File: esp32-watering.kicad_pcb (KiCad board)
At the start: 2 copper layers, 74.7 x 55.5 mm, 30 parts, among them J1 12V, J2 DS18B20, J3 FLOAT, J4 PUMP, J5 ZONE 1, J6 ZONE 2, J7 ZONE 3, K1 Pump Control, K2 Zone 1, K3 Zone 2, K4 Zone 3, Q1 2N3904, Q2 2N3904, Q3 2N3904, Q4 2N3904, U1 esp32-wemos-d1-mini, U2 TSR 1-2433

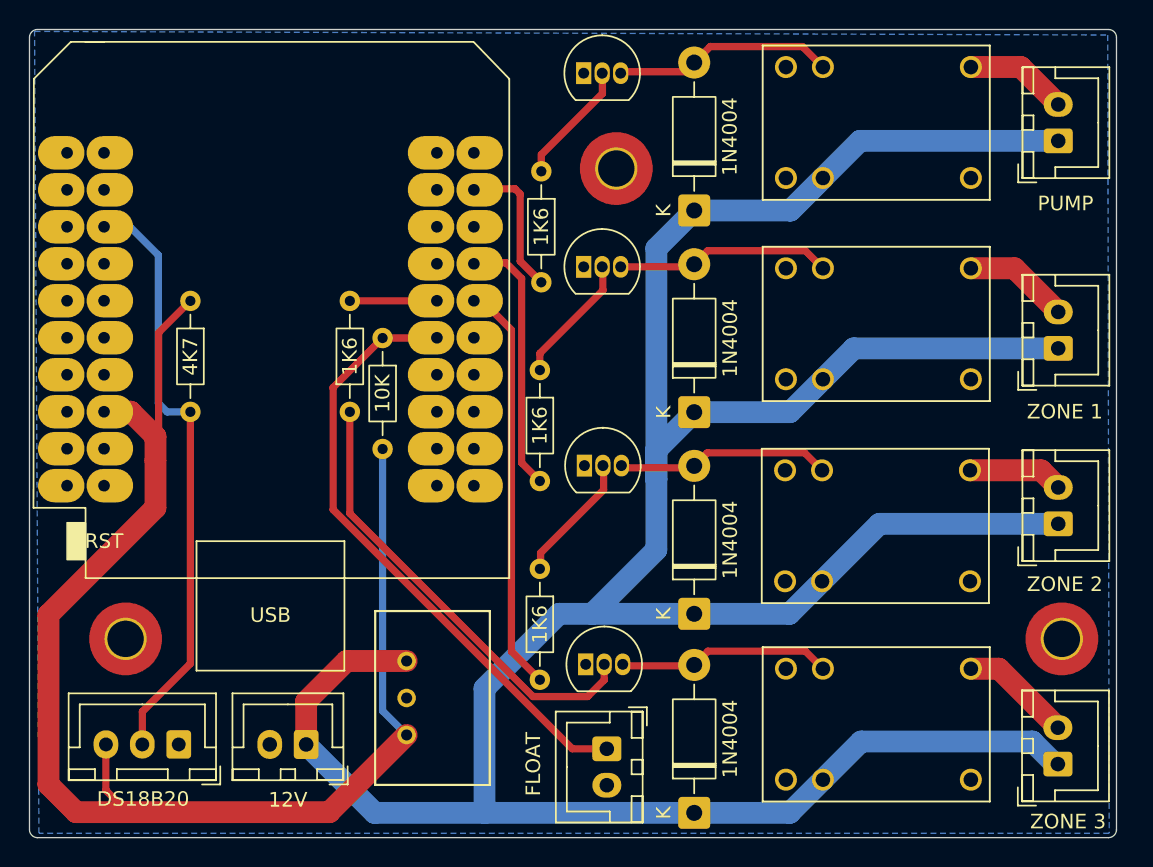
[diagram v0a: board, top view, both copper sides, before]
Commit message: Fix edge cut
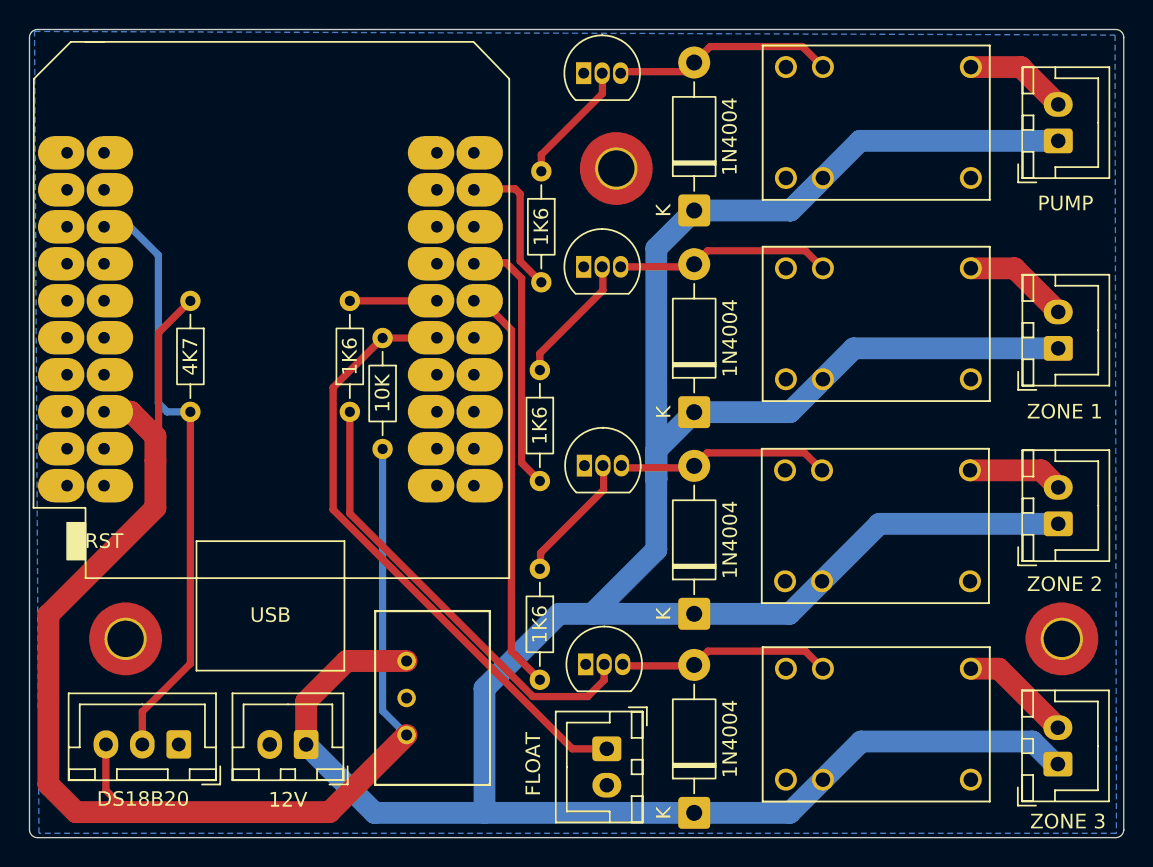
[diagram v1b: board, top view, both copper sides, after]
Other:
- board size 74.7 x 55.5 mm -> 75.2 x 55.5 mm
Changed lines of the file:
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@@
 	)
 	(gr_line
-		(start 196 80.1)
-		(end 196 25.65)
+		(start 196.5 80.1)
+		(end 196.5 25.65)
 		(stroke
 			(width 0.05)
@@
 	)
 	(gr_arc
-		(start 195.45 25.1)
-		(mid 195.838909 25.261091)
-		(end 196 25.65)
+		(start 195.95 25.1)
+		(mid 196.338909 25.261091)
+		(end 196.5 25.65)
 		(stroke
 			(width 0.05)
@@
 	(gr_line
 		(start 121.9 25.1)
-		(end 195.45 25.1)
+		(end 195.95 25.1)
 		(stroke
 			(width 0.05)
@@
 	(gr_line
 		(start 121.9 80.6)
-		(end 195.45 80.6)
+		(end 195.95 80.6)
 		(stroke
 			(width 0.05)
@@
 	)
 	(gr_arc
-		(start 196 80.05)
-		(mid 195.838909 80.438909)
-		(end 195.45 80.6)
+		(start 196.5 80.05)
+		(mid 196.338909 80.438909)
+		(end 195.95 80.6)
 		(stroke
 			(width 0.05)
@@
 		(min_thickness 0.25)
 		(filled_areas_thickness no)
-		(fill yes
+		(fill
 			(thermal_gap 0.5)
 			(thermal_bridge_width 0.5)
@@
 		(polygon
 			(pts
-				(xy 121.698715 25.232512) (xy 195.399137 25.480827) (xy 195.5 80.3) (xy 122 80.3)
+				(xy 121.698715 25.232512) (xy 195.89914 25.482512) (xy 196 80.3) (xy 122 80.3)
 			)
 		)
